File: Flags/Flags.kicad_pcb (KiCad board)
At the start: 2 copper layers, 63.5 x 41.6 mm, 28 parts, among them J1 Conn_01x07_Male, J2 Conn_01x06_Male, J3 Conn_01x03_Male, J4 Conn_01x01_Male, J5 Conn_01x01_Male, J6 Conn_01x01_Male, J7 Conn_01x01_Male, J8 Conn_01x02_Male, U1 74LS08, U2 74HC74, U3 74LS175

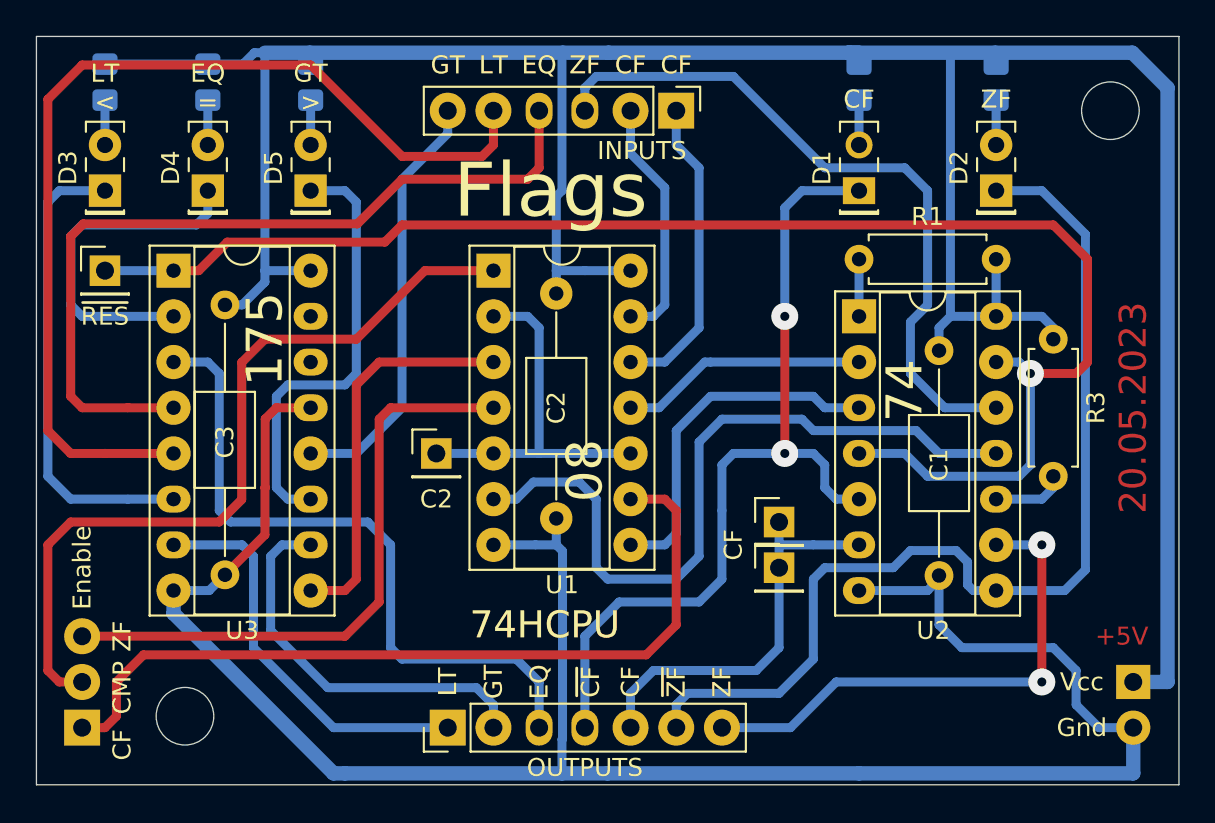
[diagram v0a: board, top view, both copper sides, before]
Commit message: Polishing Flags
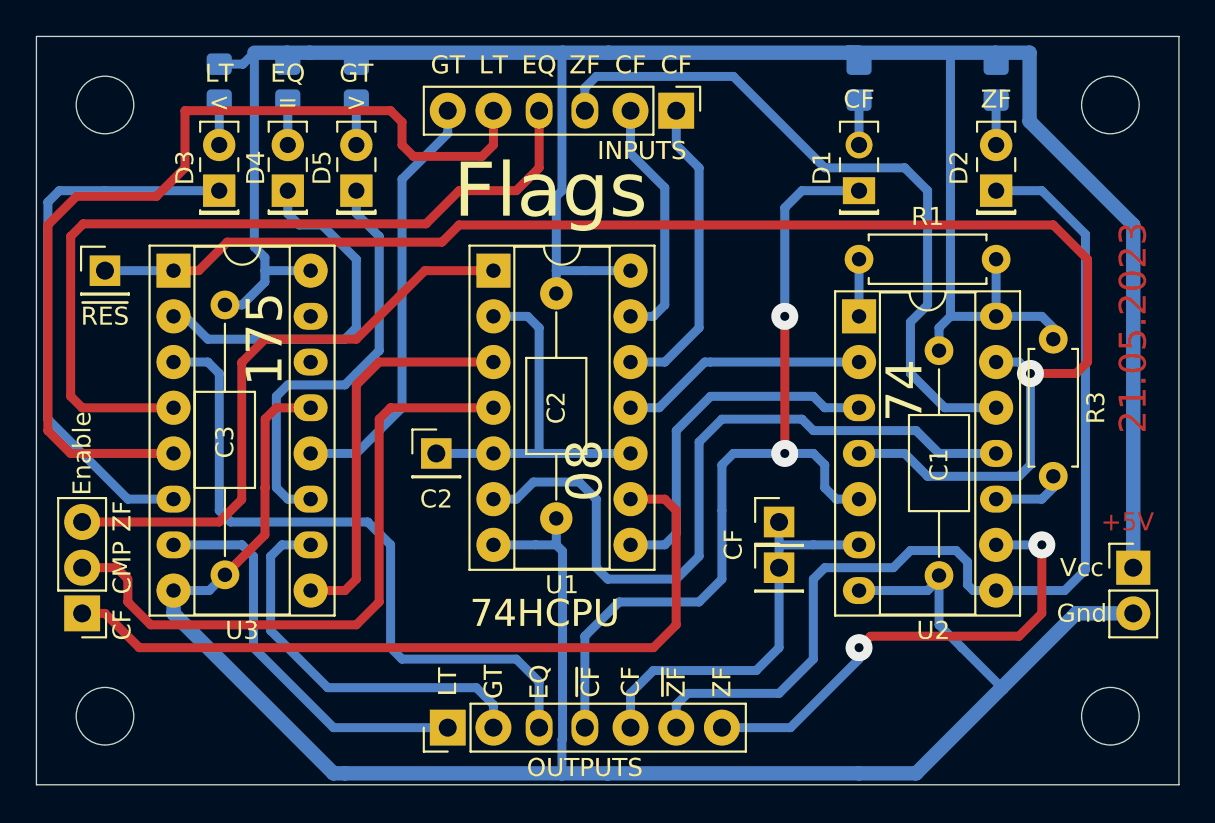
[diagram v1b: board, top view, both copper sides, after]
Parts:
- added H3: MountingHole, MountingHole:MountingHole_3.2mm_M3, F.Cu at (21.6, 21.3)
- added H4: MountingHole, MountingHole:MountingHole_3.2mm_M3, F.Cu at (77.5, 55.2)
- J3, J8: moved to F.Cu
- moved D3 6.35 mm to (27.9, 26.0)
- moved J3 6.35 mm to (20.3, 49.5), turned to 180 degrees
- moved J8 6.35 mm to (78.7, 47.0), turned to 0 degrees
- moved R5 6.35 mm to (27.9, 20.0)
- moved D4 4.45 mm to (31.8, 26.0)
- moved H2 4.45 mm to (21.6, 55.2)
- moved R6 4.45 mm to (31.8, 20.0)
- moved D5 2.54 mm to (35.6, 26.0)
- moved R7 2.54 mm to (35.6, 20.0)
- moved H1 0.32 mm to (77.5, 21.3)
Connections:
- J3 pad 2: /CMP_EN -> /ZF_EN
- J3 pad 3: /ZF_EN -> /CMP_EN
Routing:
- net VCC: track 159.9 -> 142.0 mm
- net /CMP_EN: track 44.7 -> 33.1 mm
- net GND: track 116.2 -> 108.0 mm
- net /~LT: track 26.2 -> 30.7 mm
- net /LT_IN: track 55.8 -> 52.2 mm
- net /CF_EN: track 45.7 -> 43.5 mm
- net /ZF: track 29.0 -> 27.1 mm
- net /ZF_EN: track 34.1 -> 35.9 mm
- net /~EQ: track 19.2 -> 20.9 mm
- net /~GT: track 24.5 -> 23.4 mm
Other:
- board text added: "21.05.2023"
- board text removed: "20.05.2023"
